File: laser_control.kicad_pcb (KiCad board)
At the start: 2 copper layers, 40.6 x 57.9 mm, 20 parts, among them J1 DB9, P1 CONN_01X05, Q1 BC846A, Q2 BC846A, U1 74HCT02, U2 H11L1, U3 H11L1

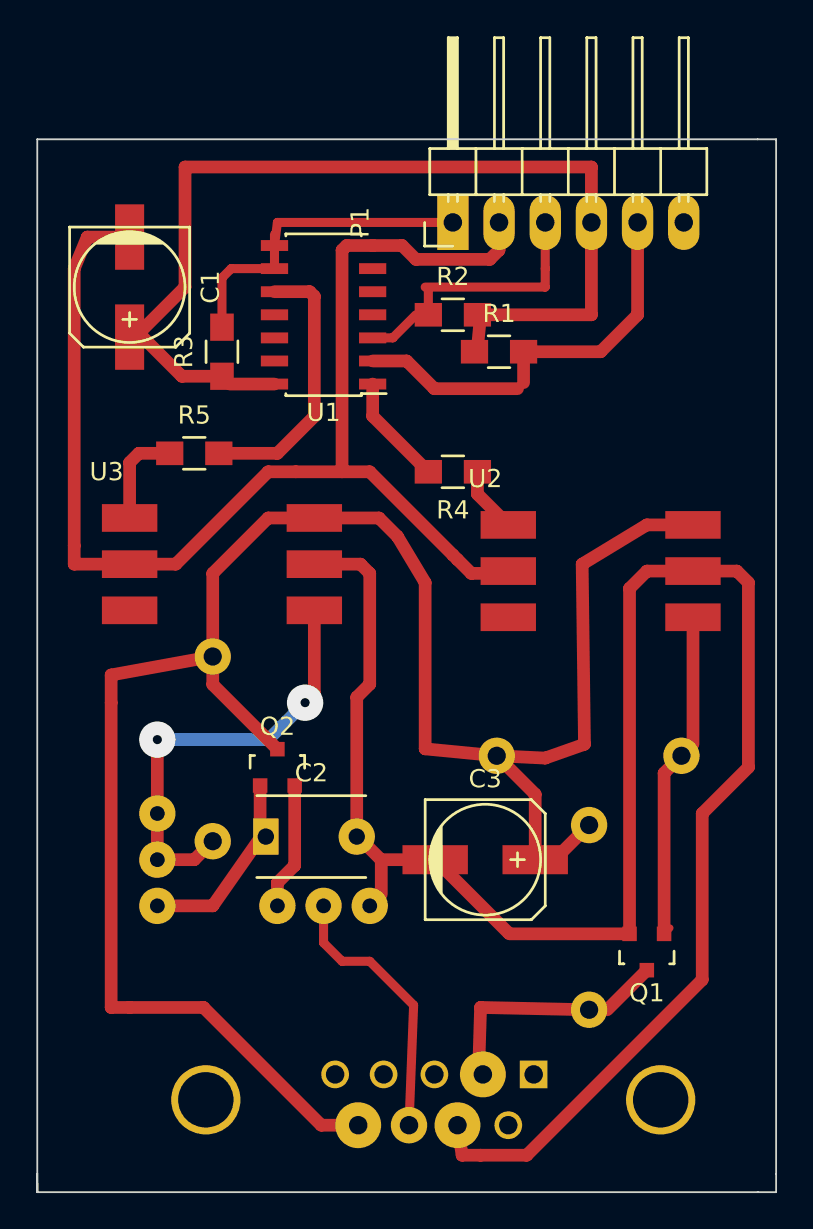
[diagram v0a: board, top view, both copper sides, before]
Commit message: Control with feedback
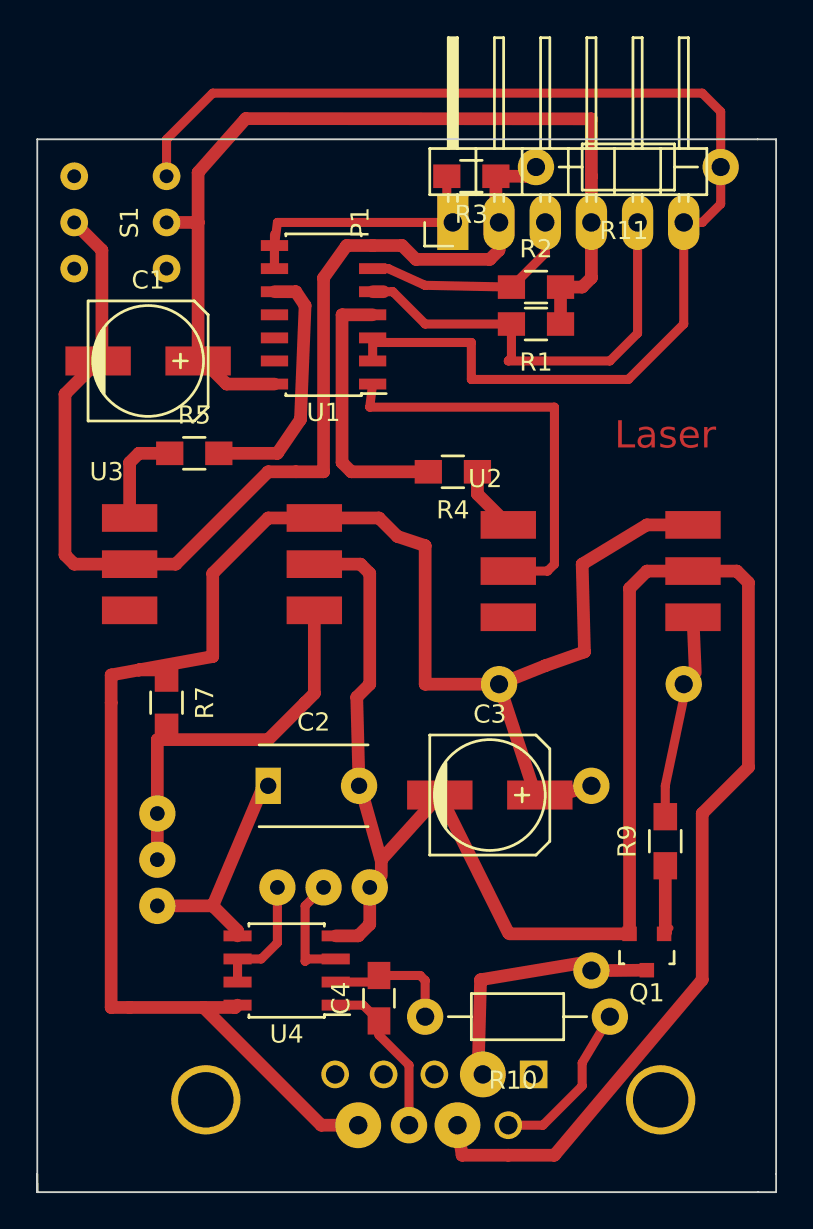
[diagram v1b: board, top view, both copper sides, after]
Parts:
- removed Q2: BC846A, TO_SOT_Packages_SMD:SOT-23
- added C4: 0.47uF, Capacitors_SMD:C_0805_HandSoldering, F.Cu at (170.7, 124.5)
- added R10: 100k, Resistors_ThroughHole:Resistor_Horizontal_RM10mm, F.Cu at (178.3, 125.5)
- added R11: 10k, Resistors_ThroughHole:Resistor_Horizontal_RM10mm, F.Cu at (184.4, 78.7)
- added R9: 4.7k, Resistors_SMD:R_0805_HandSoldering, F.Cu at (186.4, 115.8)
- added S1: button1, local:button1, F.Cu at (156.5, 81.8)
- added U4: LM358, Housings_SOIC:SOIC-8_3.9x4.9mm_Pitch1.27mm, F.Cu at (165.6, 122.9)
- R4, R5: value 220R -> 470R
- R7: footprint Resistors_ThroughHole:Resistor_Horizontal_RM10mm -> Resistors_SMD:R_0805_HandSoldering; moved to F.Cu
- moved R3 16.8 mm to (175.8, 79.2), turned to 180 degrees
- moved R2 4.82 mm to (179.3, 85.3)
- moved C1 4.19 mm to (158.0, 89.4), turned to 0 degrees
- moved R6 3.94 mm to (182.4, 107.2)
- moved R7 3.59 mm to (159.0, 108.2)
- moved C3 3.57 mm to (176.8, 113.3)
- moved C2 2.80 mm to (164.6, 112.8)
- moved R1 2.54 mm to (179.3, 87.4), turned to 180 degrees
- moved R8 2.16 mm to (182.4, 117.9)
- moved RV2 1.02 mm to (165.1, 118.4)
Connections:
- J1 pad 6: Net-(J1-Pad6) -> V_FB
- P1 pad 6: Net-(P1-Pad6) -> K+
- R3 pad 1: +5V -> GND
- R6 pad 2: Net-(Q1-Pad1) -> Net-(R6-Pad2)
- RV2 pad 2: V_REG -> Net-(RV2-Pad2)
- U1 pad 1: Net-(R4-Pad2) -> Net-(U1-Pad1)
- U1 pad 2: /K -> K+
- U1 pad 3: /P -> K+
- U1 pad 4: (no net) -> Net-(R4-Pad2)
- U1 pad 5: (no net) -> /K
- U1 pad 6: (no net) -> /P
- U2 pad 2: GND -> Net-(U1-Pad1)
- U2 pad 4: Net-(Q1-Pad1) -> Net-(R6-Pad2)
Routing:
- net K+: track 0.00 -> 68.9 mm
- net Net-(U1-Pad1): track 0.00 -> 23.0 mm
- net Net-(Q1-Pad1): track 18.5 -> 4.23 mm
- net +15V: track 112.0 -> 100.5 mm
- net Net-(R6-Pad2): track 0.00 -> 11.3 mm
- net V_FB: track 0.00 -> 9.19 mm
- net Net-(R4-Pad2): track 6.09 -> 14.8 mm
- net LASER_GND: track 106.7 -> 114.6 mm
- net GND: track 72.3 -> 65.1 mm
- net Net-(C4-Pad2): track 0.00 -> 7.18 mm
- net Net-(RV2-Pad2): track 0.00 -> 6.73 mm
- net V_REG: track 15.0 -> 9.16 mm
- net +5V: track 58.7 -> 53.1 mm
- net Net-(R7-Pad2): track 24.3 -> 20.9 mm, vias 2 -> 0
- net /P: track 15.2 -> 12.7 mm
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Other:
- net class Narrow added: clearance 0.2, trace_width 0.4, via_dia 2, via_drill 0.5
- board text added: "Laser"
